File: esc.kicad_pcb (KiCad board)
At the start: 2 copper layers, 65 parts, among them IC1 4N25, IC2 LM25101, IC3 LM25101, IC4 LM25101, IC5 ATMEGA8-AI, P1 CONN_01X03, P2 CONN_01X03, P3 CONN_01X02, P4 CONN_02X02, Q1 MOSFET_N, Q10 MOSFET_N, Q11 MOSFET_N, Q12 MOSFET_N, Q2 MOSFET_N, Q3 MOSFET_N, Q4 MOSFET_N, Q5 MOSFET_N, Q6 MOSFET_N, Q7 MOSFET_N, Q8 MOSFET_N, Q9 MOSFET_N, U1 MCP1804, U2 LM2940 10V, Y1 RESONATEUR

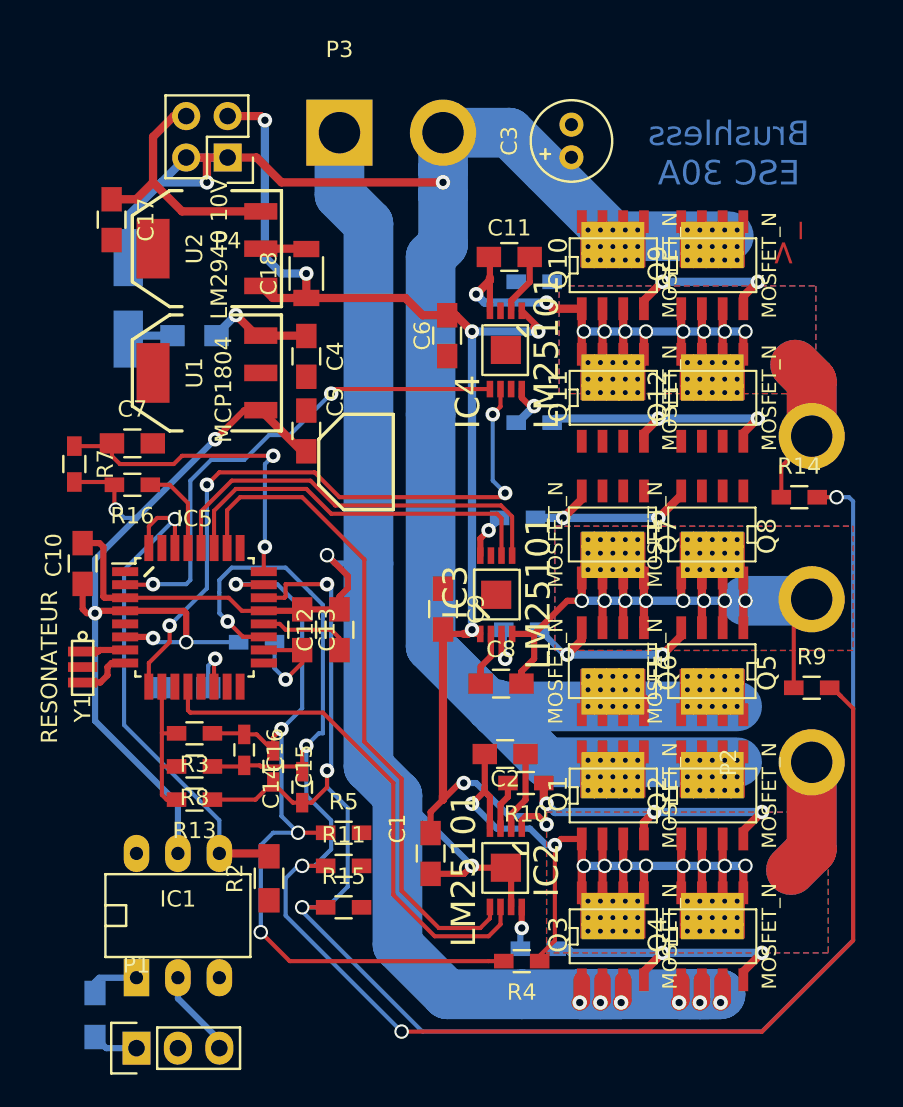
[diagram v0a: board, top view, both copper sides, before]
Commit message: PCB V1.0
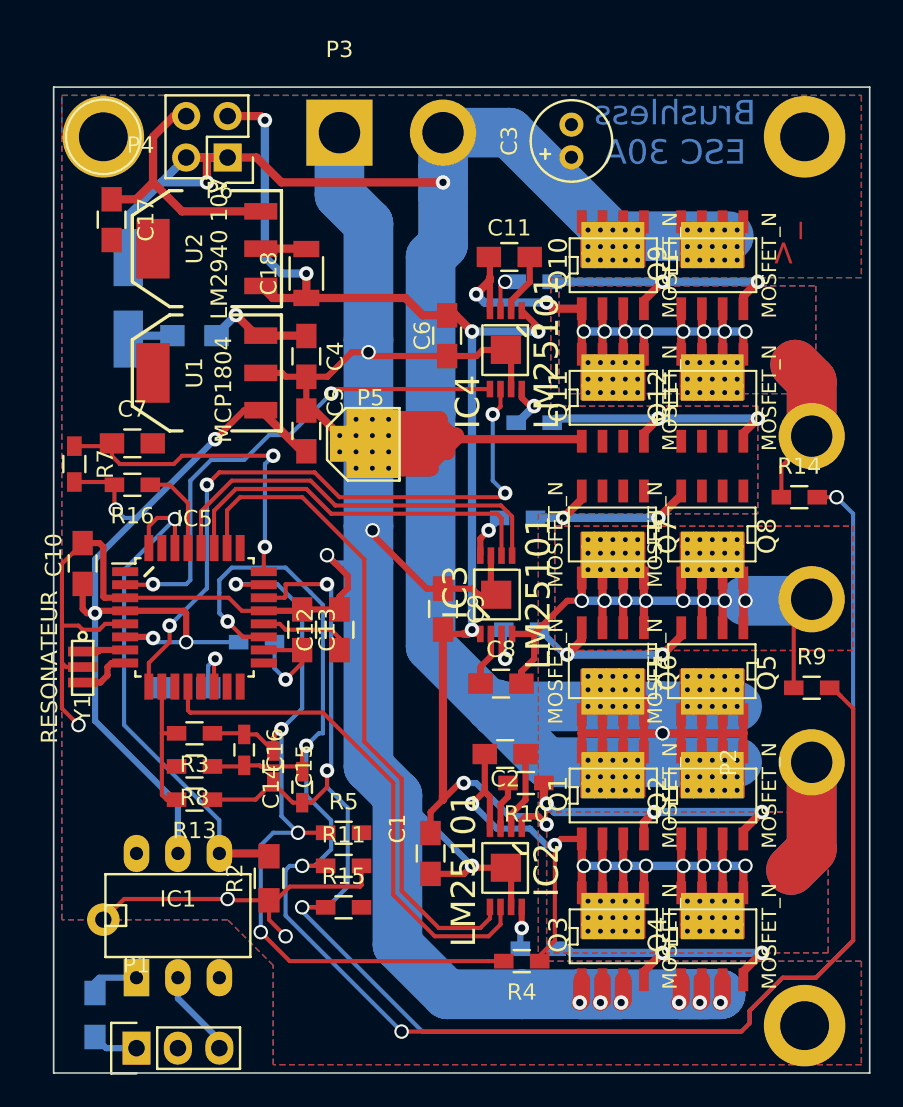
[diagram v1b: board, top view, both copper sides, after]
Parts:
- added P5: CONN_01X01, Connect:1pin, F.Cu at (204.7, 73.4)
- added P6: CONN_01X01, Connect:1pin, F.Cu at (189.2, 53.1)
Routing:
- net GND: track 144.9 -> 261.4 mm, vias 8 -> 13
- net V_BAT: track 125.1 -> 163.0 mm, vias 2 -> 3
- net /C_Highside_Gate: track 9.99 -> 16.8 mm
- net Net-(IC4-Pad3): track 0.00 -> 2.57 mm, vias 0 -> 1
- net S_B: track 102.2 -> 103.0 mm
- added copper zone on B.Cu, net GND
- added copper zone on F.Cu, net GND
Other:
- board outline added: 50 x 60.5 mm
